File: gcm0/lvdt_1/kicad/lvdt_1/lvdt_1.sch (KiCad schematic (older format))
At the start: 43 parts

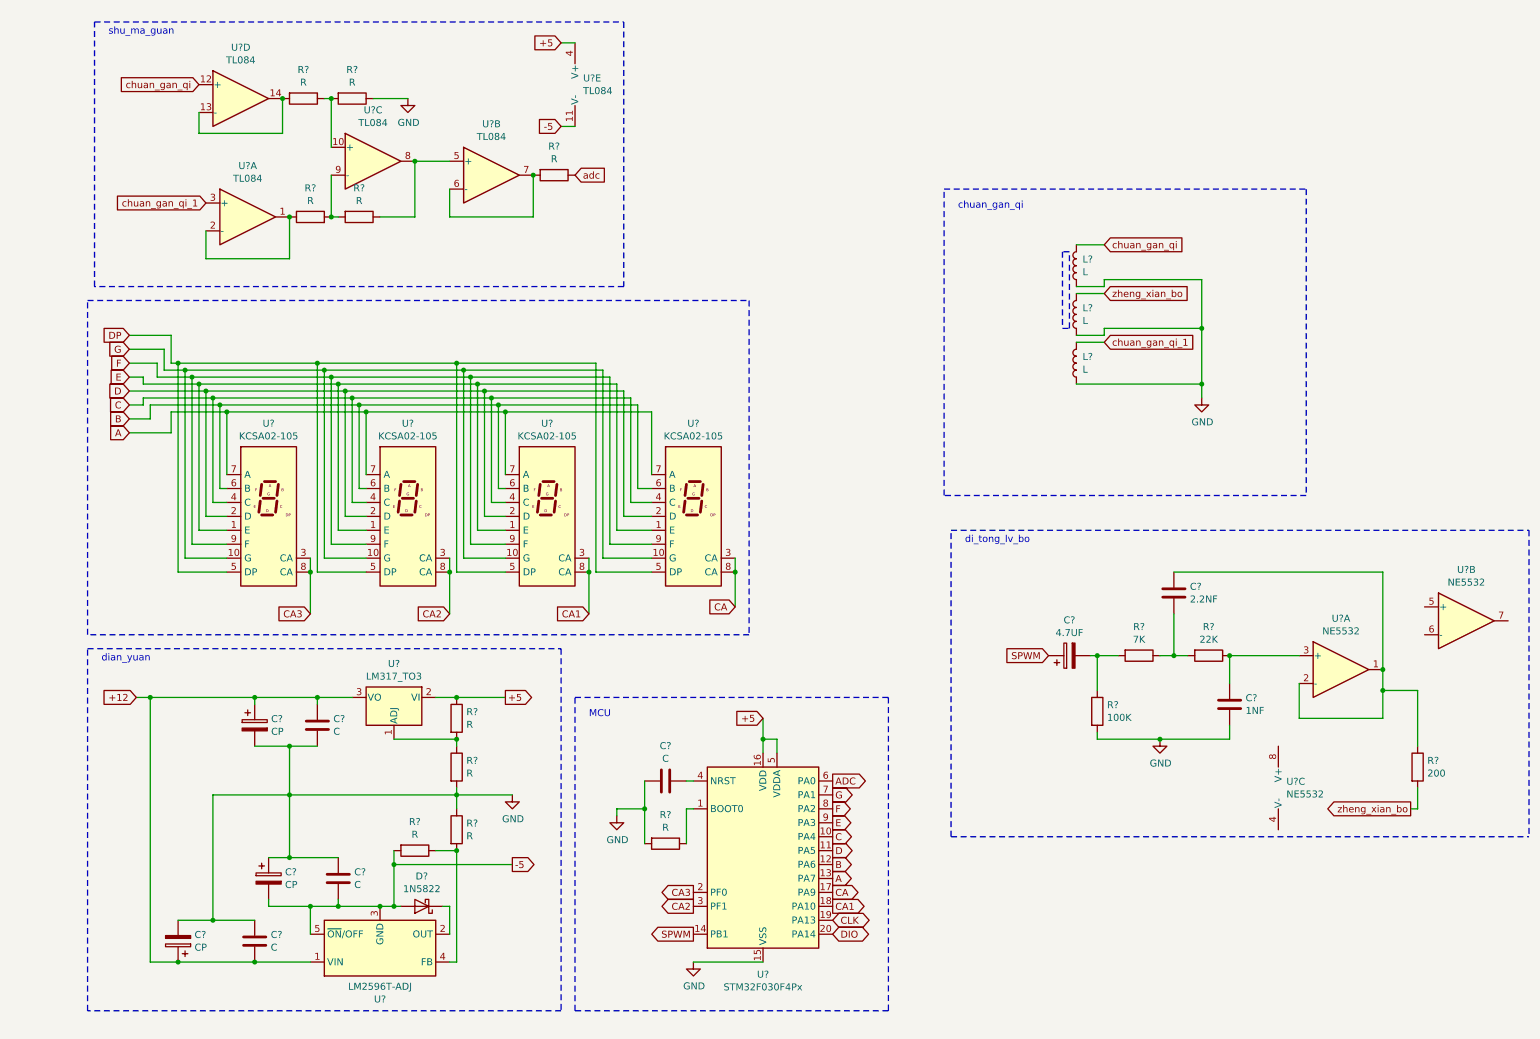
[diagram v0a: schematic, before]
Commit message: 修改原理图
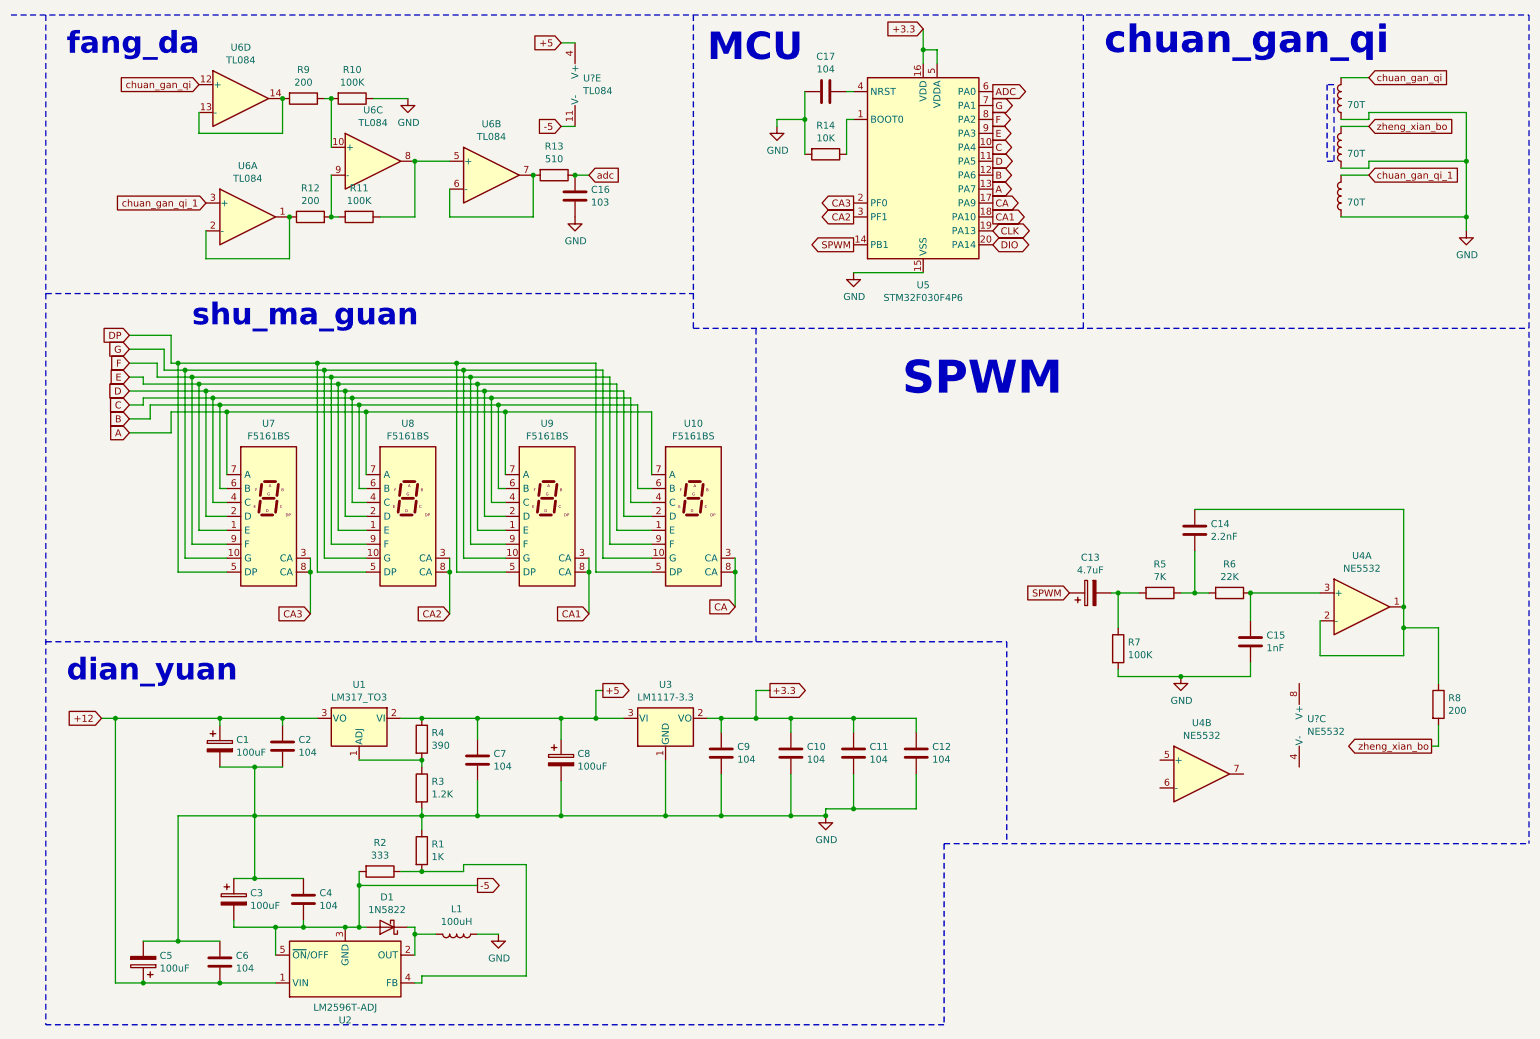
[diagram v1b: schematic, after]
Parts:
- added C10, C11, C12, C7, C9: 104, symbol Device:C
- added C16: 103, symbol Device:C
- added C8: 100uF, symbol Device:CP
- added L1: 100uH, symbol Device:L
- added U3: LM1117-3.3, symbol Regulator_Linear:LM1117-3.3
- C1, C3, C5: renamed from C?; value CP -> 100uF
- C13: renamed from C?; value 4.7UF -> 4.7uF
- C14: renamed from C?; value 2.2NF -> 2.2nF
- C15: renamed from C?; value 1NF -> 1nF
- C17, C2, C4, C6: renamed from C?; value C -> 104
- L1, L2, L3: renamed from L?; value L -> 70T
- R1: renamed from R?; value R -> 1K
- R10, R11: renamed from R?; value R -> 100K
- R12, R9: renamed from R?; value R -> 200
- R13: renamed from R?; value R -> 510
- R14: renamed from R?; value R -> 10K
- R2: renamed from R?; value R -> 333
- R3: renamed from R?; value R -> 1.2K
- R4: renamed from R?; value R -> 390
- U10, U7, U8, U9: renamed from U?; value KCSA02-105 -> F5161BS
- U5: renamed from U?; value STM32F030F4Px -> STM32F030F4P6
- gave numbers to parts that had none: 9
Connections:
- net +5: now also C7.1, C8.1, U3.3 (VI); no longer U5.16 (VDD), U5.5 (VDDA)
- net GND: now also C10.2, C11.2, C12.2, C16.2, C7.2, C8.2, C9.2, L1.1, U3.1 (GND)
- net adc: now also C16.1
- net at D1.1 (K), U2.2 (OUT): now also L1.2
- new net +3.3: C10.1, C11.1, C12.1, C9.1, U3.2 (VO), U5.16 (VDD), U5.5 (VDDA)
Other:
- note added: "SPWM"
- note added: "fang_da"
- note removed: "di_tong_lv_bo"
- moved on the sheet: C1, C13, C14, C15, C17, C2, C3, C4, C5, C6, D1, R1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
